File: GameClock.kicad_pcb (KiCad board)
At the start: 2 copper layers, 15 parts, among them J1 7-Segment-Display, SW1 SW_Push, SW2 SW_Push, SW3 SW_Push, SW4 SW_Push

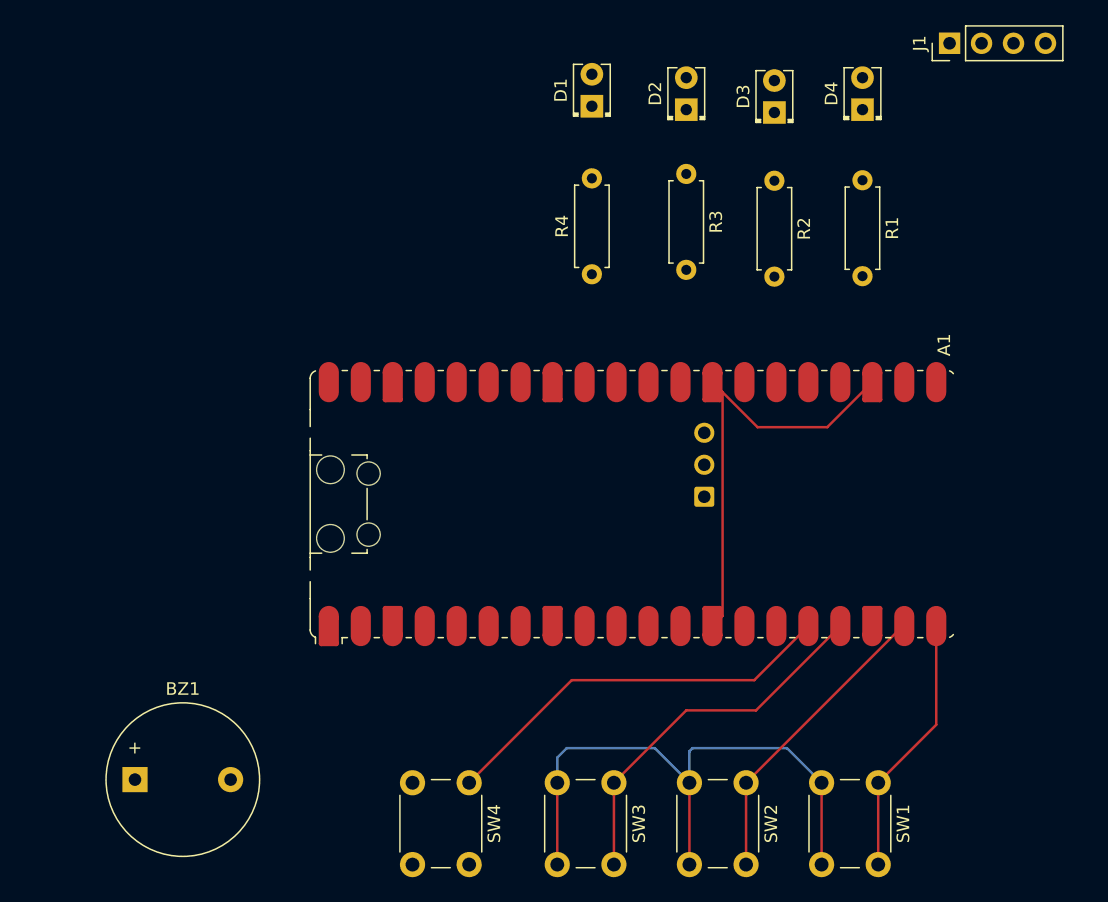
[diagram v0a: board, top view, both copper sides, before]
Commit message: finished pcbnew
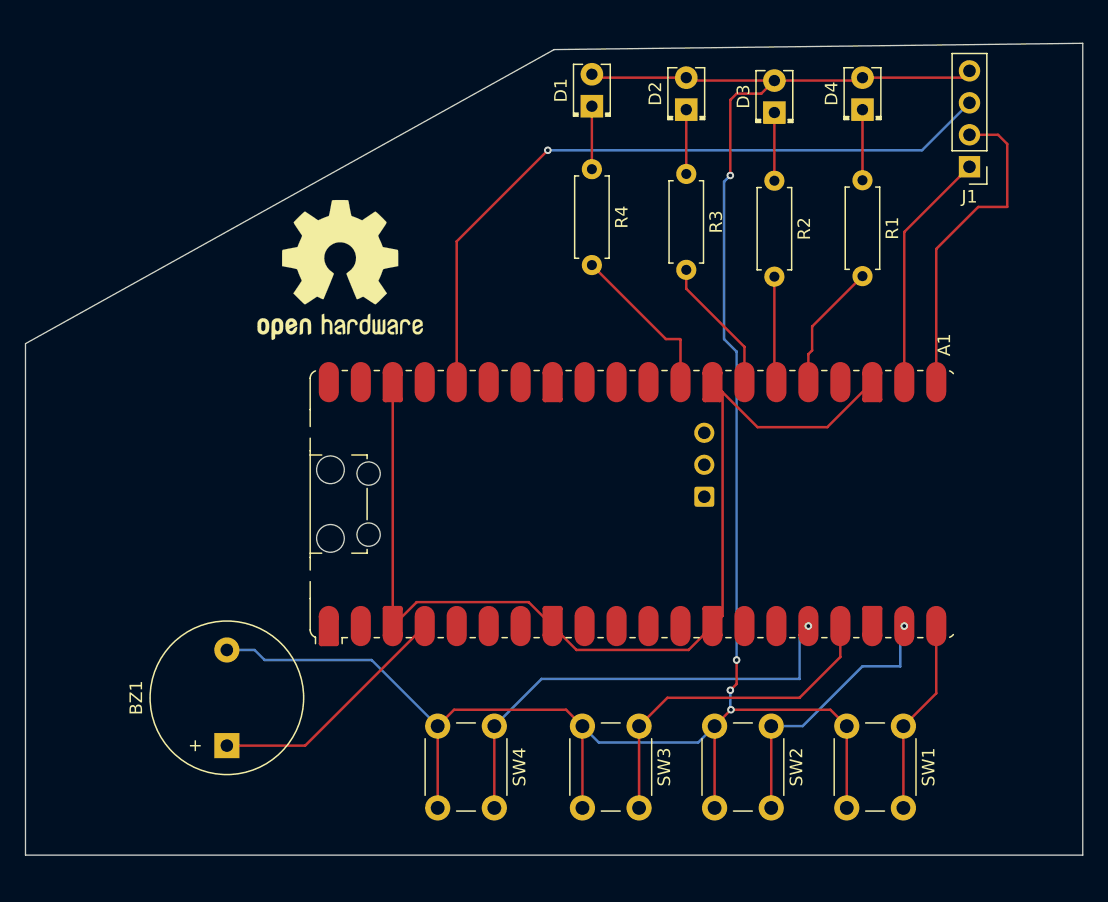
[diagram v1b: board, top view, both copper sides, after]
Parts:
- added REF**: OSHW-Logo2_14.6x12mm_SilkScreen, Symbol:OSHW-Logo2_14.6x12mm_SilkScreen, F.Cu at (209.5, 62.0)
- moved J1 9.94 mm to (259.5, 53.8), turned to 180 degrees
- moved R4 8.35 mm to (229.5, 54.0), turned to -90 degrees
- moved BZ1 7.78 mm to (200.5, 99.8), turned to 90 degrees
- moved SW1 4.92 mm to (254.2, 98.2)
- moved SW2 4.92 mm to (243.8, 98.2)
- moved SW3 4.92 mm to (233.2, 98.2)
- moved SW4 4.92 mm to (221.8, 98.2)
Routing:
- net GND: track 47.7 -> 164.9 mm, vias 0 -> 4
- net Net-(A1-3V3): track 0.00 -> 56.5 mm, vias 0 -> 1
- net Net-(A1-GND-Pad13): track 35.7 -> 83.6 mm
- net Net-(A1-GPIO16): track 0.00 -> 25.9 mm
- net Net-(A1-GPIO2): track 0.00 -> 19.7 mm
- net Net-(A1-GPIO17): track 0.00 -> 19.3 mm
- net Net-(A1-GPIO22): track 0.00 -> 12.9 mm
- net Net-(A1-GPIO21): track 0.00 -> 10.8 mm
- net Net-(A1-GPIO19): track 0.00 -> 10.2 mm
- net Net-(A1-GPIO20): track 0.00 -> 8.45 mm
- net Net-(D4-K): track 0.00 -> 5.61 mm
- net Net-(D3-K): track 0.00 -> 5.42 mm
- net Net-(A1-GPIO15): track 20.9 -> 15.5 mm
- net Net-(D2-K): track 0.00 -> 5.11 mm
- net Net-(D1-K): track 0.00 -> 5.00 mm
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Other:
- board outline added: 84 x 64.5 mm
- board text added: "AbhiramV010 Game Clock PCB"
